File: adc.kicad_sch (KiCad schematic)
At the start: 35 parts, among them U7 AD7177-2BRUZ, U70 TG2520SMN-16M-MCG, U75 OPA2189DGK

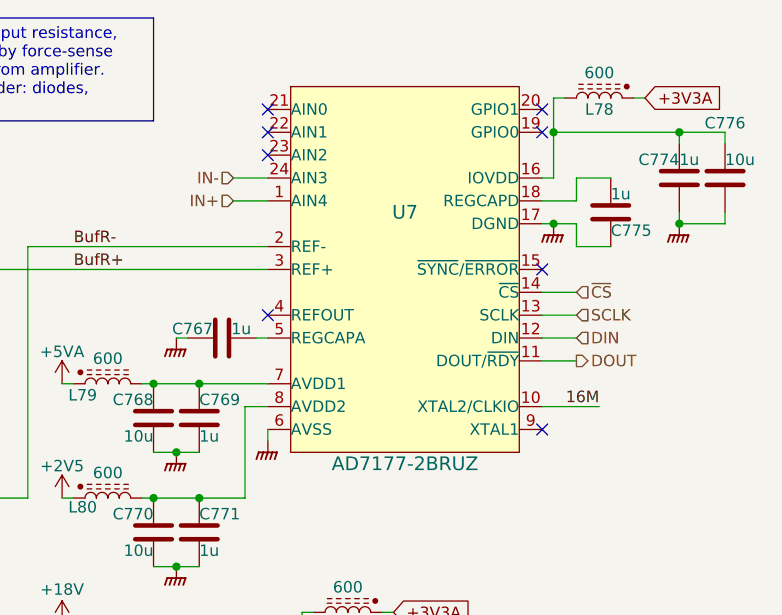
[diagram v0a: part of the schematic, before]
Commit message: Most blocks there....
About to restore scan.
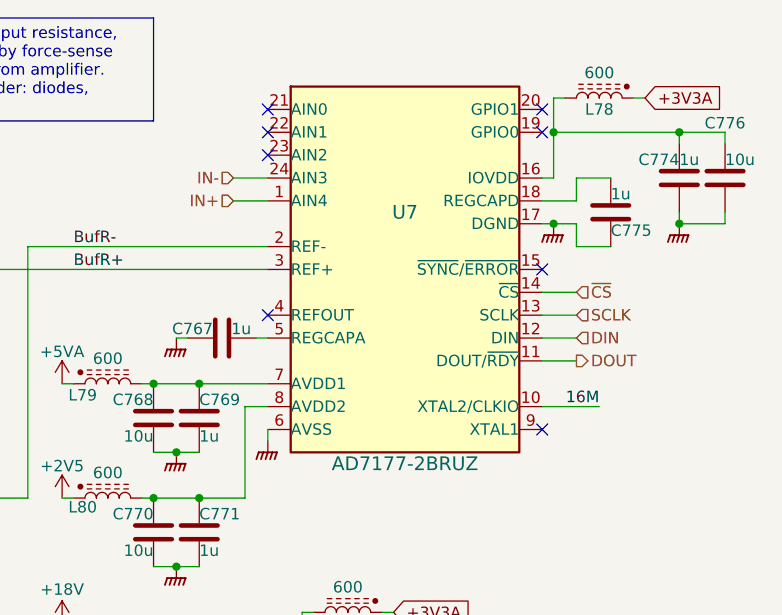
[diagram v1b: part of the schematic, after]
